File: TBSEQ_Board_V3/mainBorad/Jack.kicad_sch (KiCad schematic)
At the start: 8 parts, among them J14 Conn_01x05

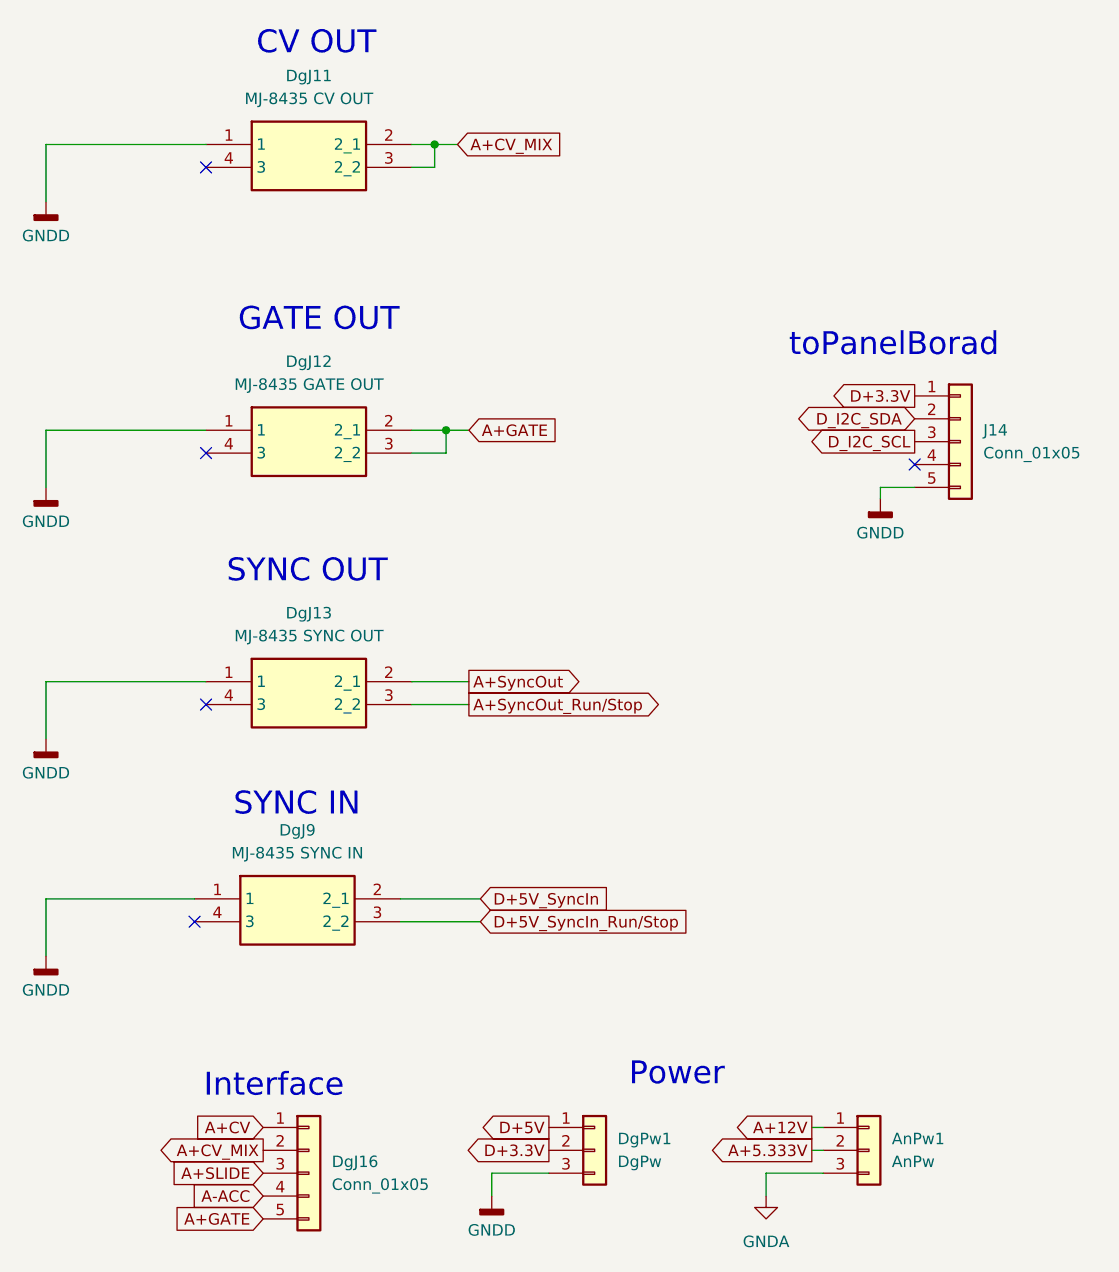
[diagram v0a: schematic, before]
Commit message: V3Board
GNDパターン塗り済
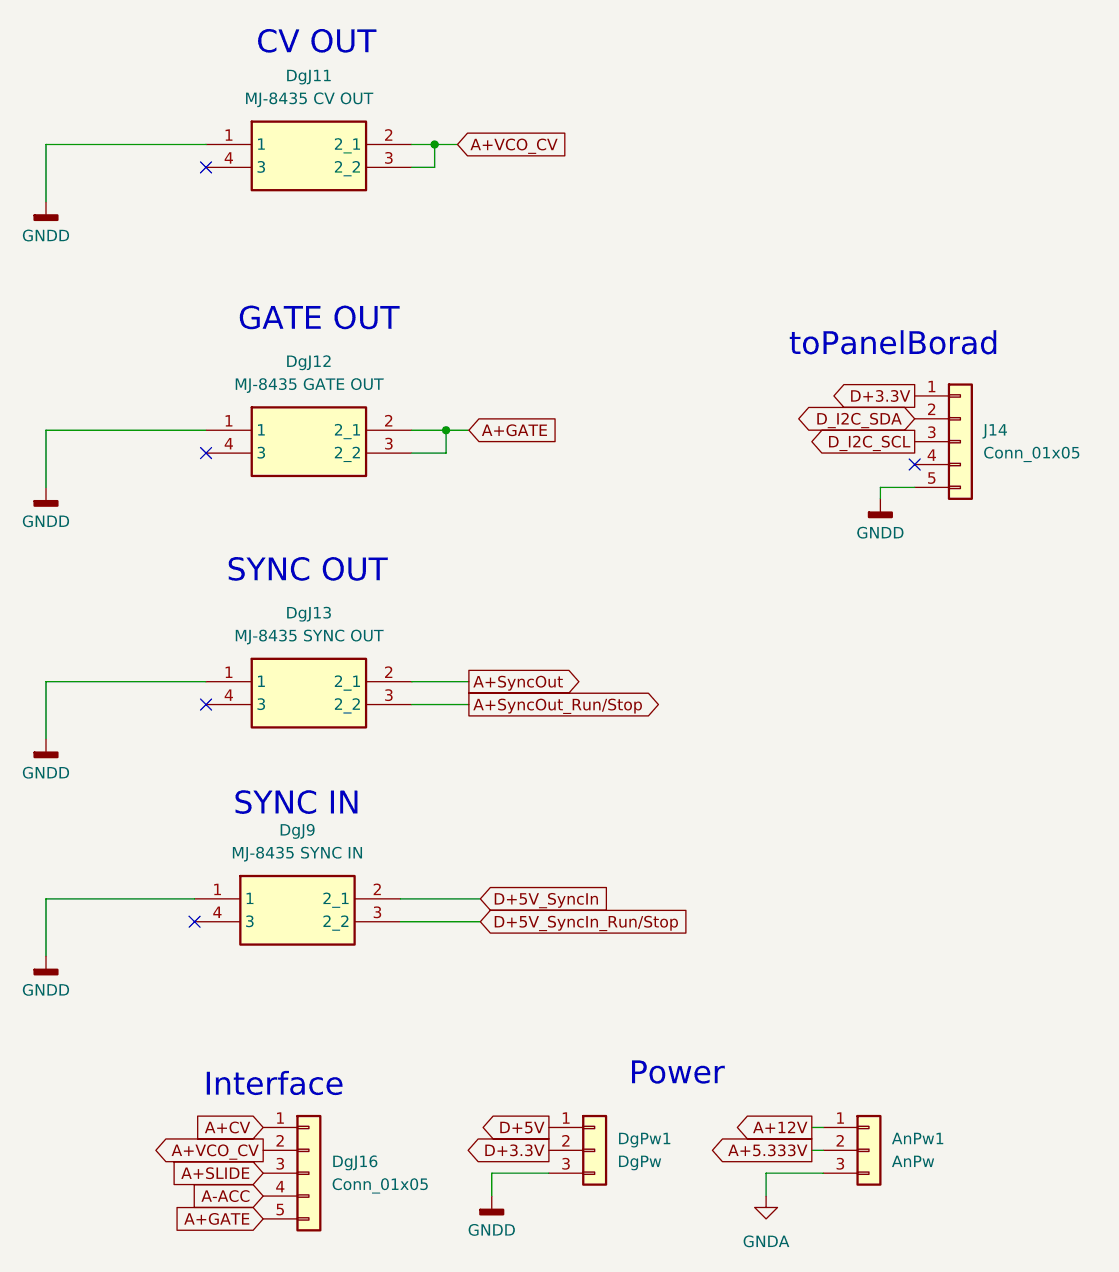
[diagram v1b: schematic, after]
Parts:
- J14: footprint Connector_JST:JST_XH_S5B-XH-A-1_1x05_P2.50mm_Horizontal -> Connector_JST:JST_XH_B5B-XH-A_1x05_P2.50mm_Vertical
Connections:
- net A+CV_MIX renamed A+VCO_CV
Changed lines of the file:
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@@
 		)
 	)
-	(global_label "A+CV_MIX"
+	(global_label "A+VCO_CV"
 		(shape output)
 		(at 104.14 143.51 180)
@@
 		)
 	)
-	(global_label "A+CV_MIX"
+	(global_label "A+VCO_CV"
 		(shape input)
 		(at 125.73 31.75 0)
@@
 			)
 		)
-		(property "Footprint" "Connector_JST:JST_XH_S5B-XH-A-1_1x05_P2.50mm_Horizontal"
+		(property "Footprint" "Connector_JST:JST_XH_B5B-XH-A_1x05_P2.50mm_Vertical"
 			(at 181.61 64.77 0)
 			(effects
